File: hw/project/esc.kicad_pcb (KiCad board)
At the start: 4 copper layers, 125 x 80 mm, 185 parts, among them J1 KFA-1016-10_16-2P, J10 I2C, J11 Misc, J12 Voltage Monitor, J2 KFA-1016-10_16-3P, J3 FTSH-107-01-L-DV-K-A, J4 Throttle, J5 Hall, J6 Serial, J7 2.54 Comm, J8 SPI, J9 CAN, Q1 SUM110P06-08L-E3, Q2 SUM110P06-08L-E3, Q3 STL110N10F7, Q4 STL110N10F7, Q5 STL110N10F7, Q6 STL110N10F7, Q7 STL110N10F7, Q8 STL110N10F7, SW1 BOOT0, SW2 RESET, SW3 USER, U1 STSPIN32G4, U2 LMR51610XDBVR, U3 ATA6561-GAQW-N, X1 SWXC5ACVF0-32.000000

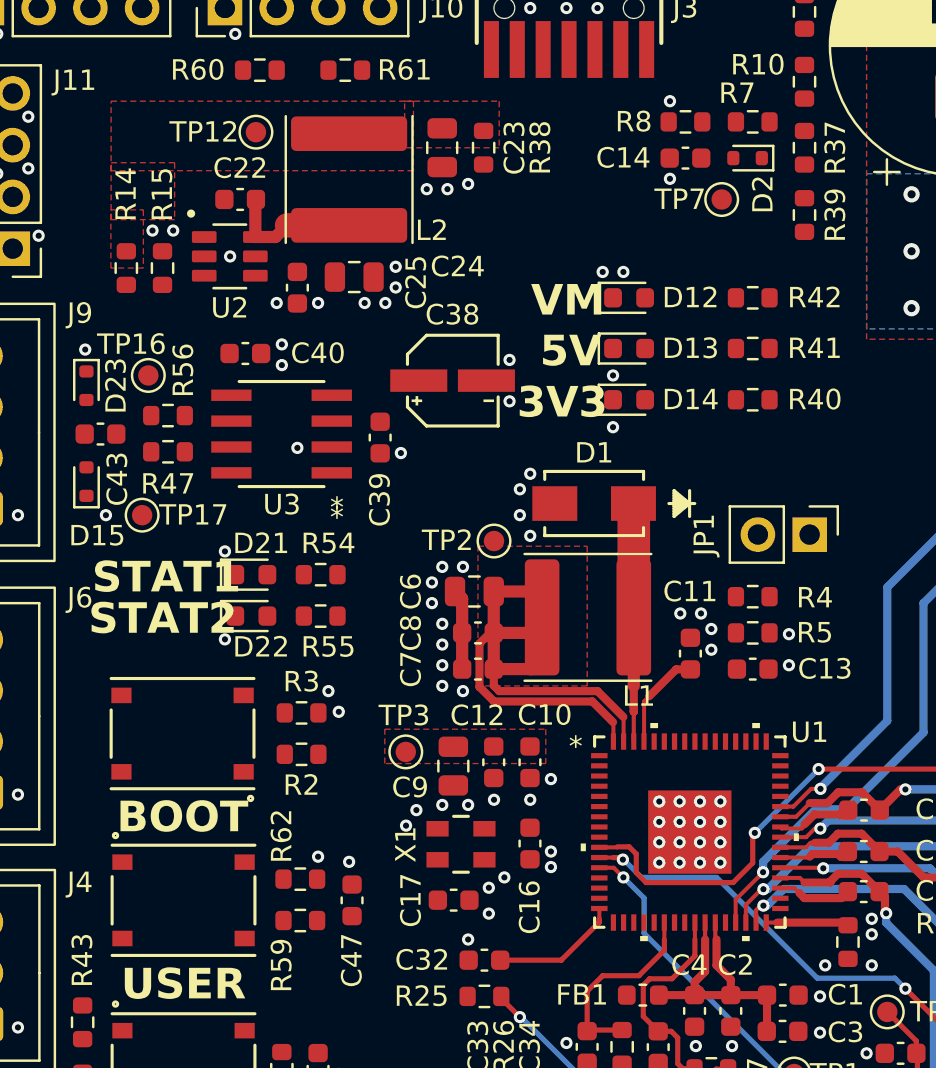
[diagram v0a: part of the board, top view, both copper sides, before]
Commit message: Route all power sections
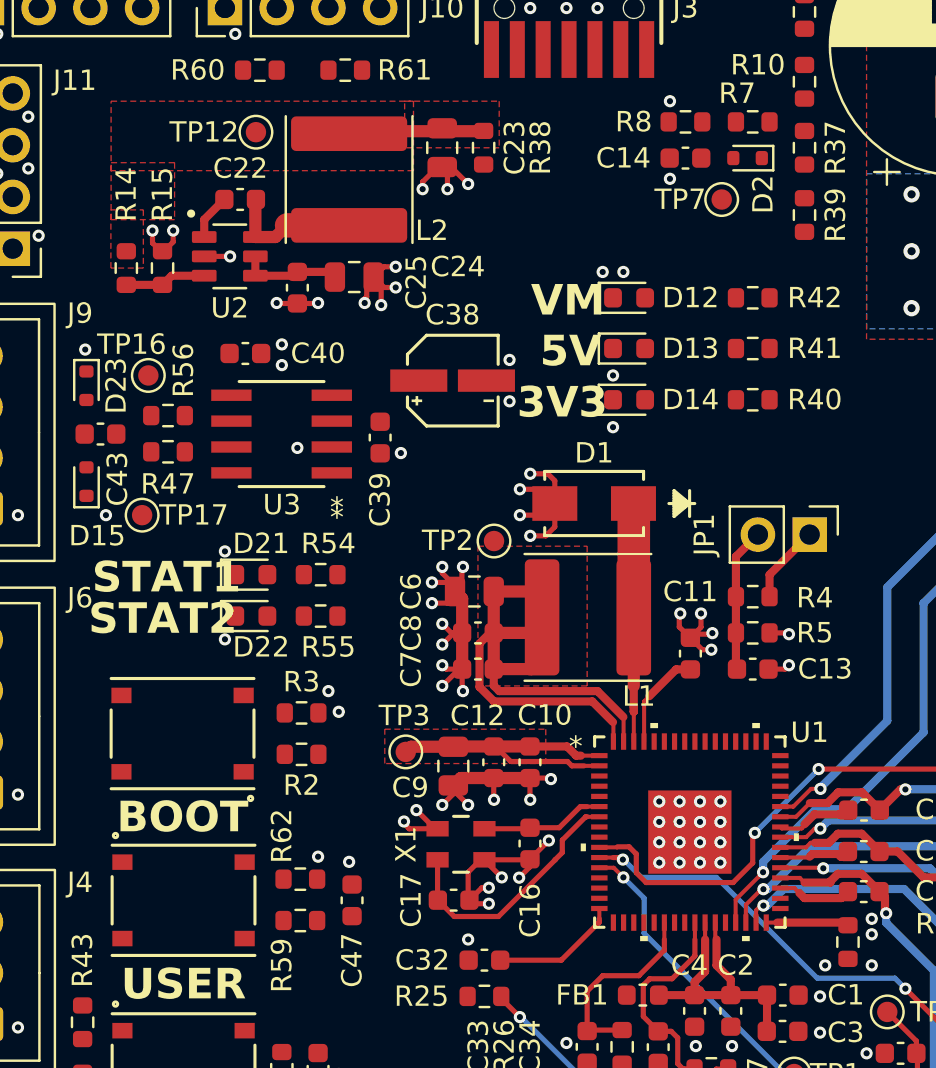
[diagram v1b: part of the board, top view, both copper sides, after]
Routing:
- net GND: track 5.43 -> 46.7 mm
- net PGND: track 32.0 -> 57.6 mm
- net VDD: track 28.7 -> 47.9 mm
- net /Control/OSC_OUT: track 0.00 -> 12.6 mm
- net /Control/SCREF: track 0.00 -> 7.07 mm
- net 5V: track 0.00 -> 6.78 mm
- net /Control/OSC_IN: track 0.00 -> 6.09 mm
- net VM: track 24.1 -> 29.1 mm
- net Net-(U2-FB): track 0.00 -> 4.01 mm
- net Net-(U2-CB): track 0.00 -> 2.34 mm
